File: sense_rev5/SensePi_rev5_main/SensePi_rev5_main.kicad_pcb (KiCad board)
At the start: 2 copper layers, 60 x 38 mm, 55 parts, among them J1 PJ-611-5A_AudioJack, J2 Conn_01x02, J3 Conn_01x06, Q1 TSM2301, Q2 Q_DUAL_NMOS_BSD840NH6327XTSA1, Q4 Q_Photo_NPN, SW1 SW_SPST, SW2 Slider_Switch_SW_2_State, U1 MDBT42Q, U2 MCP4012T-503E/CH, U3 TLV8802, U4 PIR, Y1 Crystal

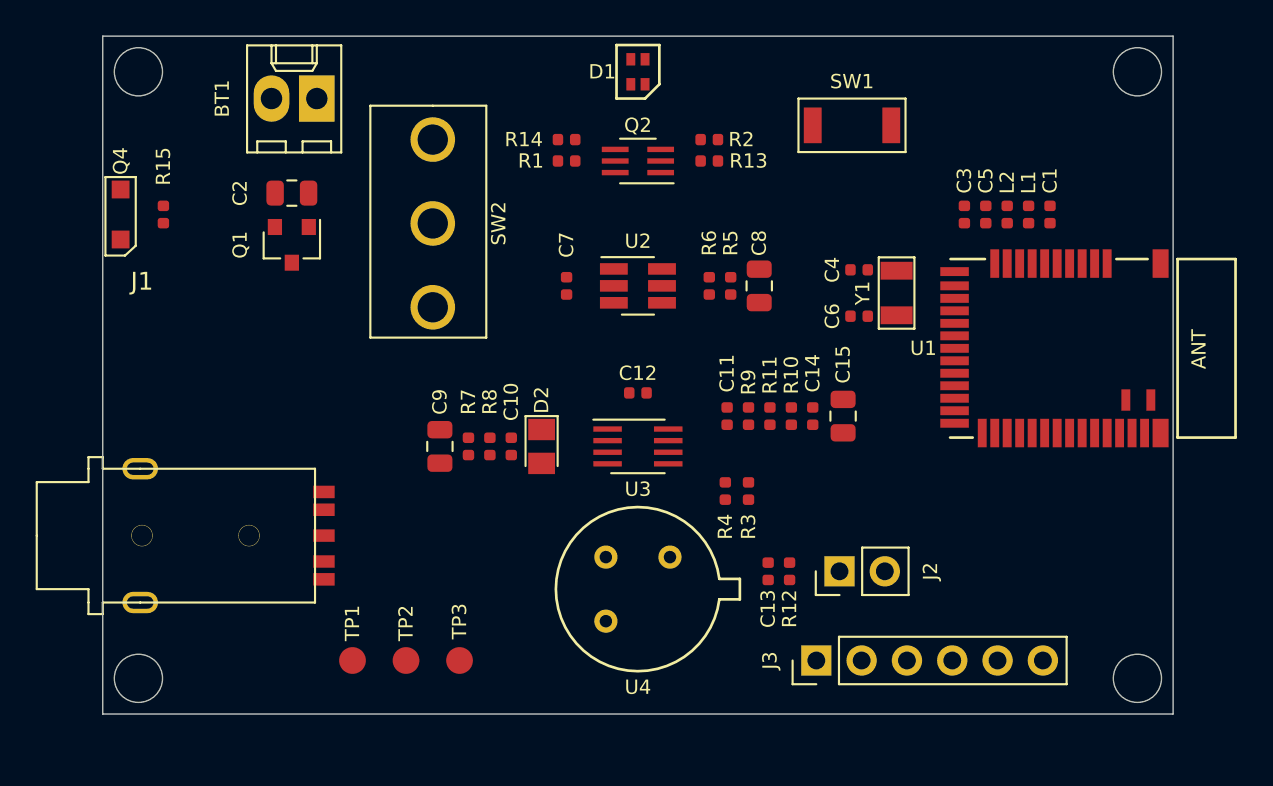
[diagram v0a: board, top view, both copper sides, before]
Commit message: sense_rev5 PCB Design files completed.
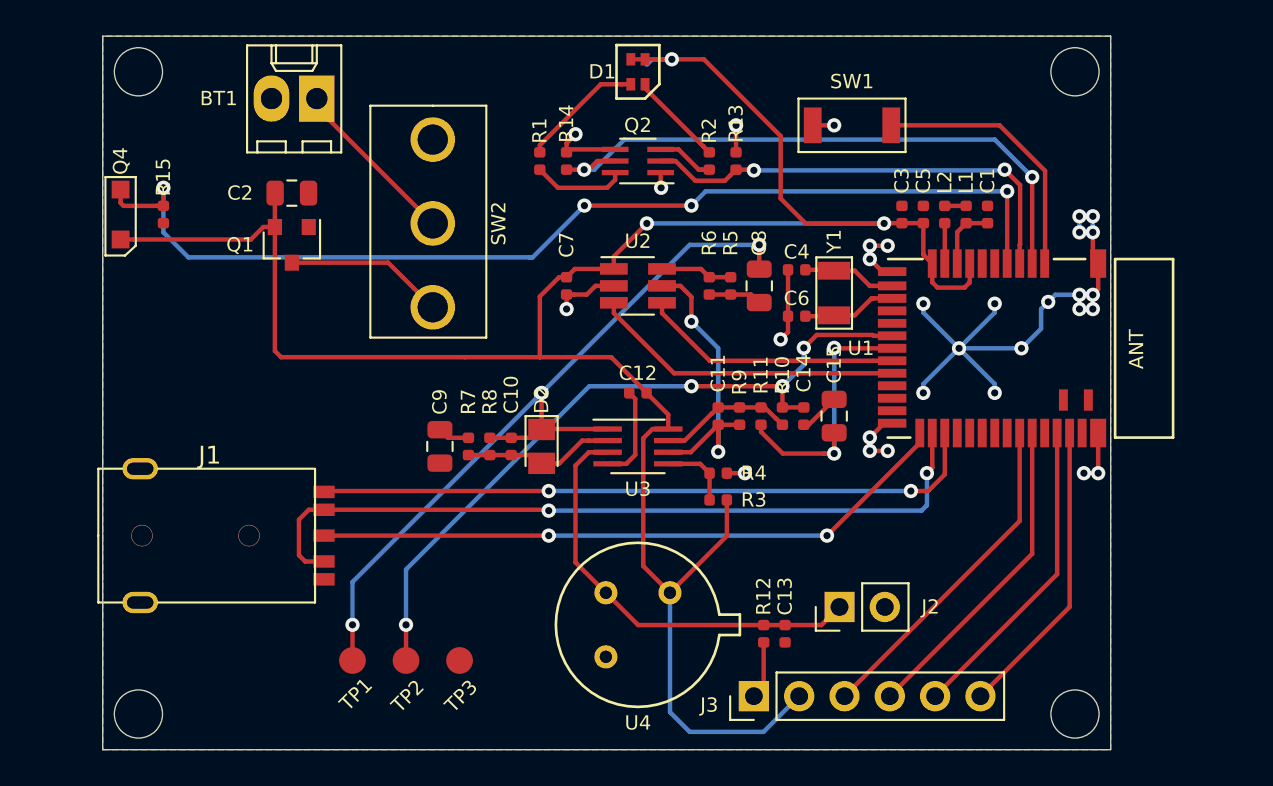
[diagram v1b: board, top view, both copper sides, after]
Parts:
- moved J3 4.03 mm to (46.5, 47.0)
- moved MK2 4.03 mm to (64.5, 48.0)
- moved R12 3.79 mm to (47.0, 43.5), turned to 270 degrees
- moved C13 3.63 mm to (48.2, 43.5), turned to 270 degrees
- moved C1 3.50 mm to (59.6, 20.0)
- moved C3 3.50 mm to (54.8, 20.0)
- moved C4 3.50 mm to (48.9, 23.1)
- moved C5 3.50 mm to (56.0, 20.0)
- moved C6 3.50 mm to (48.9, 25.7)
- moved L1 3.50 mm to (58.4, 20.0)
- moved L2 3.50 mm to (57.2, 20.0)
- moved MK3 3.50 mm to (64.5, 12.0)
- moved U1 3.50 mm to (60.5, 27.5)
- moved Y1 3.50 mm to (51.0, 24.4)
- moved J2 2.00 mm to (51.3, 42.0)
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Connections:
- net /GPIO2 renamed Net-(U1-Pad32)
- J3 pad 5: /SWDIO -> /SWDCLK
- J3 pad 6: /SWDCLK -> /SWDIO
- U1 pad 31: /RX -> Net-(U1-Pad31)
- U1 pad 33: /GPIO1 -> /RX
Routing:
- net VDD: track 0.00 -> 130.7 mm, vias 0 -> 3
- net GND: track 0.00 -> 69.9 mm, vias 0 -> 30
- net /LED_SENSE: track 0.00 -> 60.3 mm, vias 0 -> 4
- net /OUT_A: track 0.00 -> 45.2 mm, vias 0 -> 3
- net /FOCUS: track 0.00 -> 43.3 mm, vias 0 -> 2
- net /AMP_SIGNAL: track 0.00 -> 40.8 mm, vias 0 -> 4
- net /TRIGGER: track 0.00 -> 37.5 mm, vias 0 -> 2
- net /AUDIO_JACK_IO: track 0.00 -> 36.1 mm, vias 0 -> 2
- net /LED_GREEN: track 0.00 -> 34.5 mm, vias 0 -> 2
- net /LED_RED: track 0.00 -> 25.7 mm, vias 0 -> 2
- net /PIR_OUT: track 0.00 -> 24.2 mm
- net /RX: track 0.00 -> 18.8 mm
- net /TX: track 0.00 -> 18.1 mm
- net /SWDCLK: track 0.00 -> 17.6 mm
- net /MCP4012T_U\D: track 0.00 -> 17.6 mm
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- added copper zone on B.Cu, net GND
- added copper zone on F.Cu, net GND
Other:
- board size 60 x 38 mm -> 56.5 x 40 mm
